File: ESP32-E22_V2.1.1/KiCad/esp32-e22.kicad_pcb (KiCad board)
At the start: 2 copper layers, 70 x 99 mm, 42 parts, among them J1 Conn_01x02_Socket, J10 Conn_01x02_Socket, J3 Screw_Terminal_01x02, J4 Conn_01x04_Socket, J5 Conn_01x03_Socket, J6 Conn_01x04_Socket, J7 Conn_01x05_Socket, J8 SMA, J9 Conn_01x02_Socket, SW1 SW_Push, U1 ESP32-DevKitC, U2 DM-OLED096-636, U3 E22-40033S

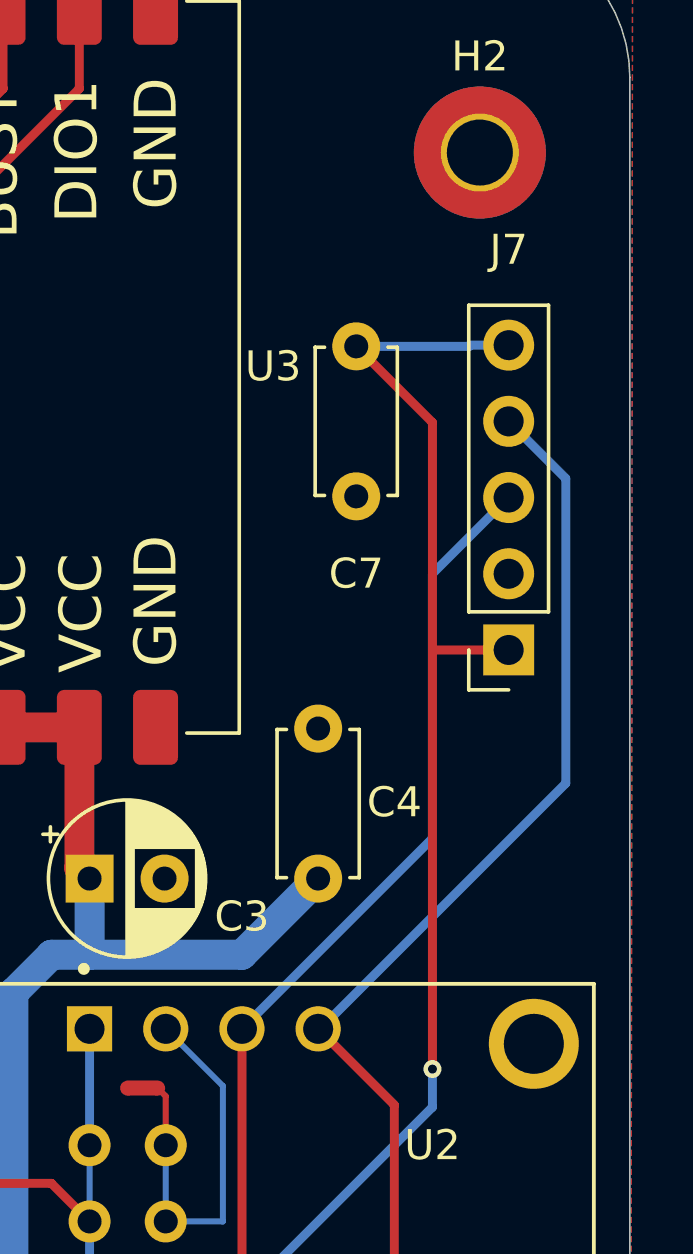
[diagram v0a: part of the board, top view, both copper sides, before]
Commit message: Update esp32-e22.kicad_pcb
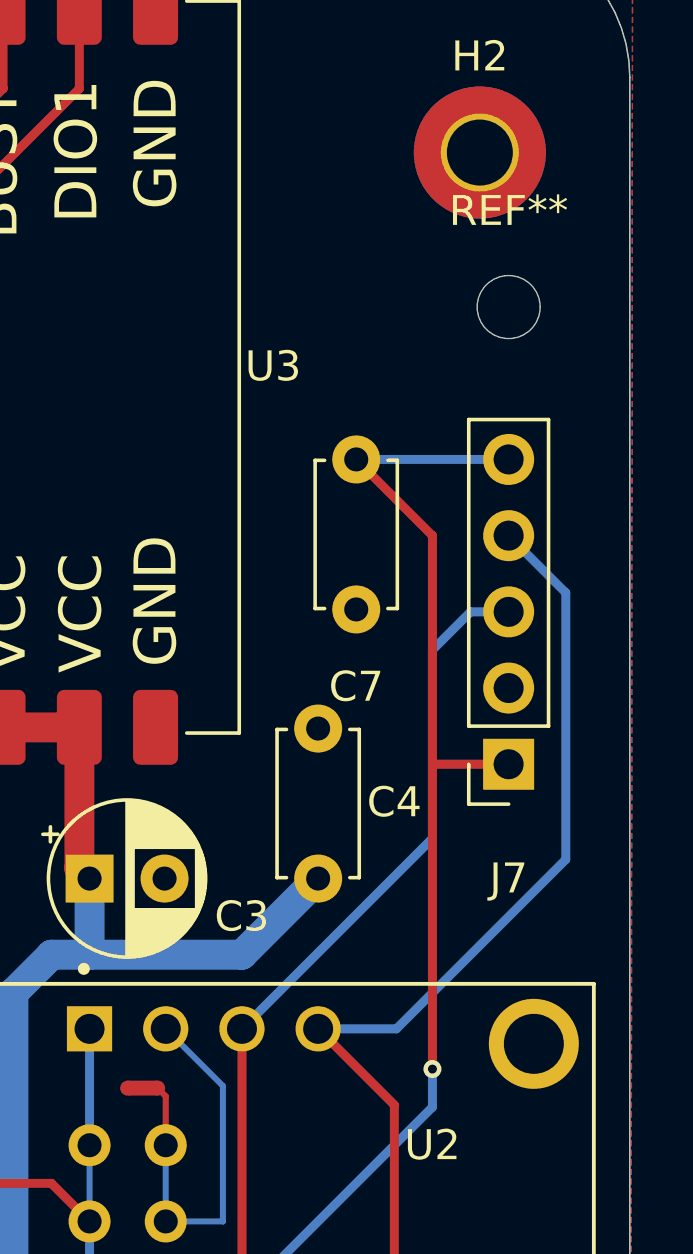
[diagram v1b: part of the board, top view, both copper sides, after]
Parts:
- added REF**: MountingHole_2.1mm, MountingHole:MountingHole_2.1mm, F.Cu at (176.5, 68.6)
- moved J7 3.81 mm to (176.5, 83.8)
- moved C7 3.77 mm to (171.4, 73.7)
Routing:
- net +3.3V: track 185.5 -> 181.8 mm
- net /SCL: track 110.5 -> 107.5 mm
- net /SDA: track 129.1 -> 126.7 mm
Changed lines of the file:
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@@
 	(footprint "Connector_PinSocket_2.54mm:PinSocket_1x05_P2.54mm_Vertical"
 		(layer "F.Cu")
-		(at 176.53 80.01 180)
+		(at 176.53 83.82 180)
 		(descr "Through hole straight socket strip, 1x05, 2.54mm pitch, single row (from Kicad 4.0.7), script generated")
 		(tags "Through hole socket strip THT 1x05 2.54mm single row")
 		(property "Reference" "J7"
-			(at 0 13.335 360)
+			(at 0 -3.81 0)
 			(layer "F.SilkS")
 			(effects
@@
 		)
 		(property "Value" "Conn_01x05_Socket"
-			(at 0 12.93 360)
+			(at 0 12.93 0)
 			(layer "F.Fab")
 			(effects
@@
 		)
 	)
+	(footprint "MountingHole:MountingHole_2.1mm"
+		(layer "F.Cu")
+		(at 176.53 68.58)
+		(descr "Mounting Hole 2.1mm, no annular")
+		(tags "mounting hole 2.1mm no annular")
+		(property "Reference" "REF**"
+			(at 0 -3.2 0)
+			(layer "F.SilkS")
+			(effects
+				(font
+					(size 1 1)
+					(thickness 0.15)
+				)
+			)
+		)
+		(property "Value" "MountingHole_2.1mm"
+			(at 0 3.2 0)
+			(layer "F.Fab")
+			(effects
+				(font
+					(size 1 1)
+					(thickness 0.15)
+				)
+			)
+		)
+		(property "Footprint" "MountingHole:MountingHole_2.1mm"
+			(at 0 0 0)
+			(unlocked yes)
+			(layer "F.Fab")
+			(hide yes)
+			(effects
+				(font
+					(size 1.27 1.27)
+					(thickness 0.15)
+				)
+			)
+		)
+		(property "Datasheet" ""
+			(at 0 0 0)
+			(unlocked yes)
+			(layer "F.Fab")
+			(hide yes)
+			(effects
+				(font
+					(size 1.27 1.27)
+					(thickness 0.15)
+				)
+			)
+		)
+		(property "Description" ""
+			(at 0 0 0)
+			(unlocked yes)
+			(layer "F.Fab")
+			(hide yes)
+			(effects
+				(font
+					(size 1.27 1.27)
+					(thickness 0.15)
+				)
+			)
+		)
+		(attr exclude_from_pos_files exclude_from_bom)
+		(fp_circle
+			(center 0 0)
+			(end 2.1 0)
+			(stroke
+				(width 0.15)
+				(type solid)
+			)
+			(fill none)
+			(layer "Cmts.User")
+		)
+		(fp_circle
+			(center 0 0)
+			(end 2.35 0)
+			(stroke
+				(width 0.05)
+				(type solid)
+			)
+			(fill none)
+			(layer "F.CrtYd")
+		)
+		(fp_text user "${REFERENCE}"
+			(at 0 0 0)
+			(layer "F.Fab")
+			(effects
+				(font
+					(size 1 1)
+					(thickness 0.15)
+				)
+			)
+		)
+		(pad "" np_thru_hole circle
+			(at 0 0)
+			(size 2.1 2.1)
+			(drill 2.1)
+			(layers "*.Cu" "*.Mask")
+		)
+	)
 	(footprint "Capacitor_THT:CP_Radial_D5.0mm_P2.50mm"
 		(layer "F.Cu")
@@
 	(footprint "Capacitor_THT:C_Disc_D4.7mm_W2.5mm_P5.00mm"
 		(layer "F.Cu")
-		(at 171.45 69.89 -90)
+		(at 171.45 73.66 -90)
 		(descr "C, Disc series, Radial, pin pitch=5.00mm, , diameter*width=4.7*2.5mm^2, Capacitor, http://www.vishay.com/docs/45233/krseries.pdf")
 		(tags "C Disc series Radial pin pitch 5.00mm  diameter 4.7mm width 2.5mm Capacitor")
@@
 	)
 	(segment
-		(start 127 96.52)
-		(end 128.27 97.79)
-		(width 0.3)
-		(layer "F.Cu")
-		(net 2)
-	)
-	(segment
-		(start 124.46 96.52)
-		(end 127 96.52)
+		(start 173.99 93.98)
+		(end 173.99 76.2)
 		(width 0.3)
 		(layer "F.Cu")
@@
 	)
 	(segment
-		(start 173.99 80.01)
-		(end 173.99 72.43)
+		(start 173.99 76.2)
+		(end 171.45 73.66)
 		(width 0.3)
 		(layer "F.Cu")
@@
 	)
 	(segment
-		(start 173.99 80.01)
-		(end 176.53 80.01)
+		(start 127 96.52)
+		(end 128.27 97.79)
 		(width 0.3)
 		(layer "F.Cu")
@@
 	)
 	(segment
-		(start 128.27 97.79)
-		(end 161.29 97.79)
+		(start 124.46 96.52)
+		(end 127 96.52)
 		(width 0.3)
 		(layer "F.Cu")
@@
 	)
 	(segment
-		(start 173.99 93.98)
-		(end 173.99 80.01)
+		(start 173.99 83.82)
+		(end 176.53 83.82)
 		(width 0.3)
 		(layer "F.Cu")
@@
 	)
 	(segment
-		(start 173.99 72.43)
-		(end 171.45 69.89)
+		(start 128.27 97.79)
+		(end 161.29 97.79)
 		(width 0.3)
 		(layer "F.Cu")
@@
 	)
 	(segment
-		(start 176.53 69.85)
-		(end 175.26 69.85)
-		(width 0.3)
-		(layer "B.Cu")
-		(net 2)
-	)
-	(segment
 		(start 118.11 95.25)
 		(end 119.38 95.25)
@@
 	)
 	(segment
-		(start 175.22 69.89)
-		(end 171.45 69.89)
-		(width 0.3)
-		(layer "B.Cu")
-		(net 2)
-	)
-	(segment
 		(start 118.11 101.6)
 		(end 118.11 95.25)
@@
 	)
 	(segment
+		(start 176.53 73.66)
+		(end 171.45 73.66)
+		(width 0.3)
+		(layer "B.Cu")
+		(net 2)
+	)
+	(segment
 		(start 116.84 114.3)
 		(end 115.57 113.03)
@@
 	)
 	(segment
-		(start 175.26 69.85)
-		(end 175.22 69.89)
-		(width 0.3)
-		(layer "B.Cu")
-		(net 2)
-	)
-	(segment
 		(start 122.555 130.165)
 		(end 122.555 115.291346)
@@
 	)
 	(segment
-		(start 178.435 74.295)
-		(end 176.53 72.39)
+		(start 178.435 86.995)
+		(end 178.435 78.105)
 		(width 0.3)
 		(layer "B.Cu")
@@
 	)
 	(segment
-		(start 178.435 84.455)
-		(end 178.435 74.295)
+		(start 172.79 92.64)
+		(end 178.435 86.995)
 		(width 0.3)
 		(layer "B.Cu")
@@
 	)
 	(segment
-		(start 170.18 92.64)
-		(end 170.25 92.64)
+		(start 178.435 78.105)
+		(end 176.53 76.2)
 		(width 0.3)
 		(layer "B.Cu")
@@
 	)
 	(segment
-		(start 170.25 92.64)
-		(end 178.435 84.455)
+		(start 170.18 92.64)
+		(end 172.79 92.64)
 		(width 0.3)
 		(layer "B.Cu")
@@
 	)
 	(segment
+		(start 173.99 80.01)
+		(end 175.26 78.74)
+		(width 0.3)
+		(layer "B.Cu")
+		(net 6)
+	)
+	(segment
 		(start 167.64 92.64)
 		(end 173.99 86.29)
@@
 	(segment
 		(start 173.99 86.29)
-		(end 173.99 77.47)
+		(end 173.99 80.01)
 		(width 0.3)
 		(layer "B.Cu")
@@
 	)
 	(segment
-		(start 173.99 77.47)
-		(end 176.53 74.93)
+		(start 175.26 78.74)
+		(end 176.53 78.74)
 		(width 0.3)
 		(layer "B.Cu")
